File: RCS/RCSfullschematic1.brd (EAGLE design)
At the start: 102.5 x 80 mm, 67 parts, among them IC1 ILD213T, IC2 FT232RL, IC4 317T, J7 USB-MICROB, Q2 8 MHz, T1 MMBT2222A, U1 MPL3115A2, U2 MPU-9250, U3 ATMEGA328P_TQFP, U4 ADS1015

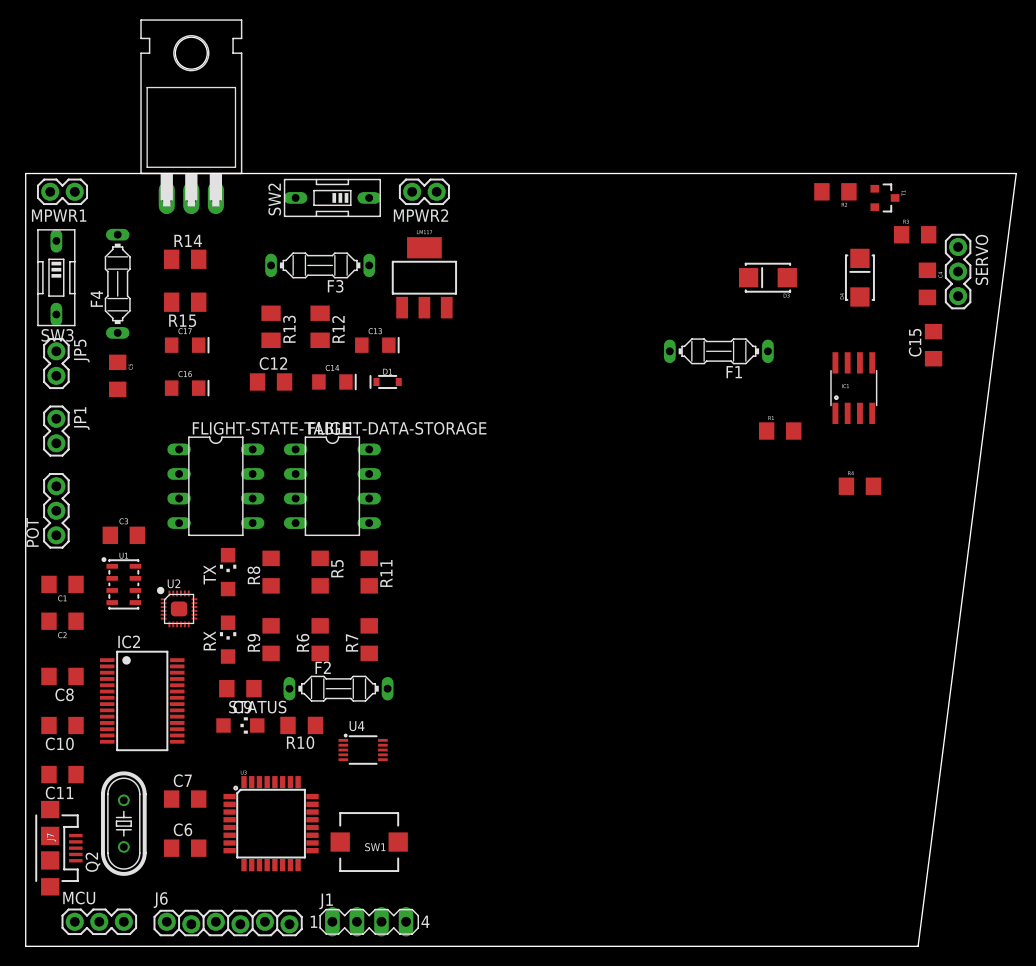
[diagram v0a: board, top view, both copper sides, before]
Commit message: Small Update to board
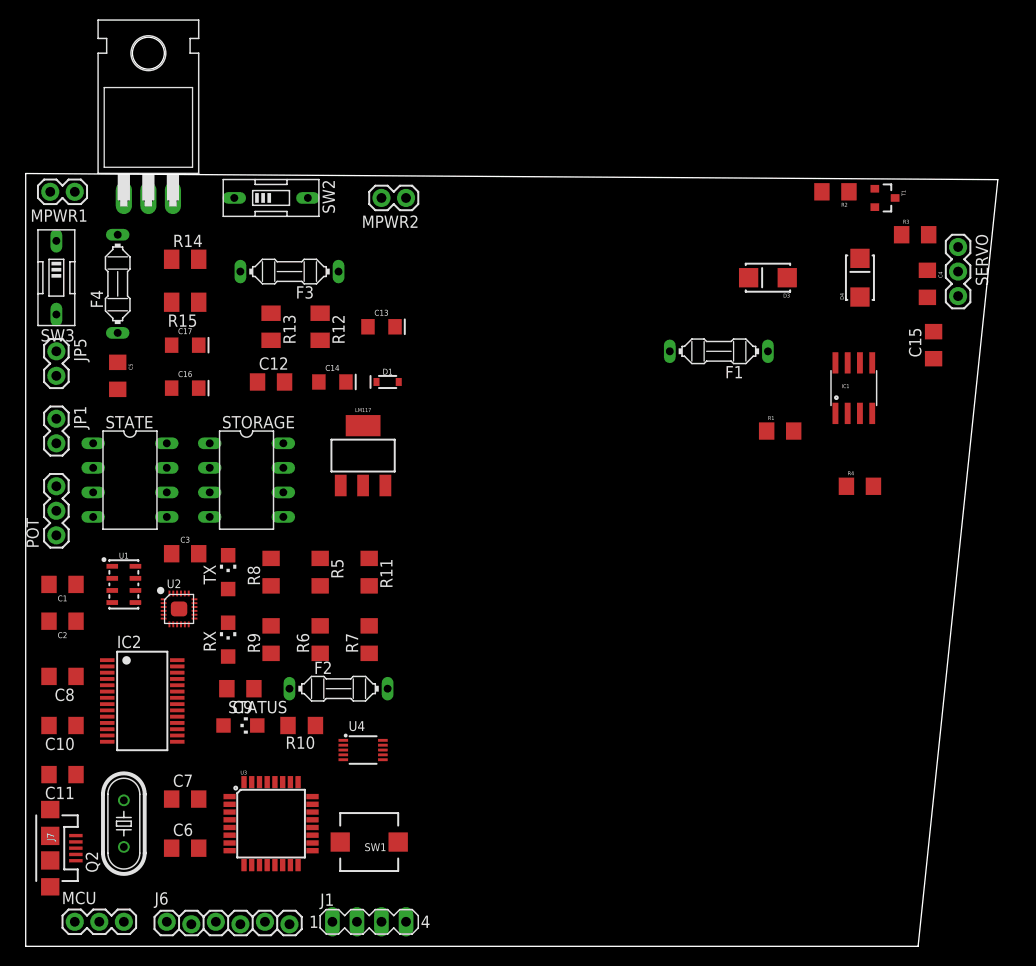
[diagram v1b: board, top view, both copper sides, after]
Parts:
- removed FLIGHT-DATA-STORAGE, FLIGHT-STATE-TABLE: AT24CP, atmel:DIL08
- added STATE, STORAGE: AT24CP, atmel:DIL08
- moved LM117 19.5 mm to (34.9, 50.8)
- moved C3 6.63 mm to (16.5, 40.6)
- moved SW2 6.35 mm to (25.4, 77.5), turned to 270 degrees
- moved IC4 4.45 mm to (12.7, 87.6)
- moved MPWR2 3.24 mm to (39.4, 77.5)
- moved F3 3.24 mm to (27.3, 69.8)
- moved C13 2.01 mm to (36.8, 64.1)
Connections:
- net A4(SDA): now also STATE.5, STORAGE.5; no longer FLIGHT-DATA-STORAGE.5, FLIGHT-STATE-TABLE.5
- net A5(SCL): now also STATE.6, STORAGE.6; no longer FLIGHT-DATA-STORAGE.6, FLIGHT-STATE-TABLE.6
- net GND: now also STATE.1, STATE.2, STATE.4, STORAGE.1, STORAGE.2, STORAGE.3, STORAGE.4, STORAGE.7; no longer FLIGHT-DATA-STORAGE.1, FLIGHT-DATA-STORAGE.2, FLIGHT-DATA-STORAGE.3, FLIGHT-DATA-STORAGE.4, FLIGHT-DATA-STORAGE.7, FLIGHT-STATE-TABLE.1, FLIGHT-STATE-TABLE.2, FLIGHT-STATE-TABLE.4
- net VCC: now also STATE.3, STATE.7, STATE.8, STORAGE.8; no longer FLIGHT-DATA-STORAGE.8, FLIGHT-STATE-TABLE.3, FLIGHT-STATE-TABLE.7, FLIGHT-STATE-TABLE.8
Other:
- board size 102.5 x 80 mm -> 100.6 x 80 mm

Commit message: yayyyyy
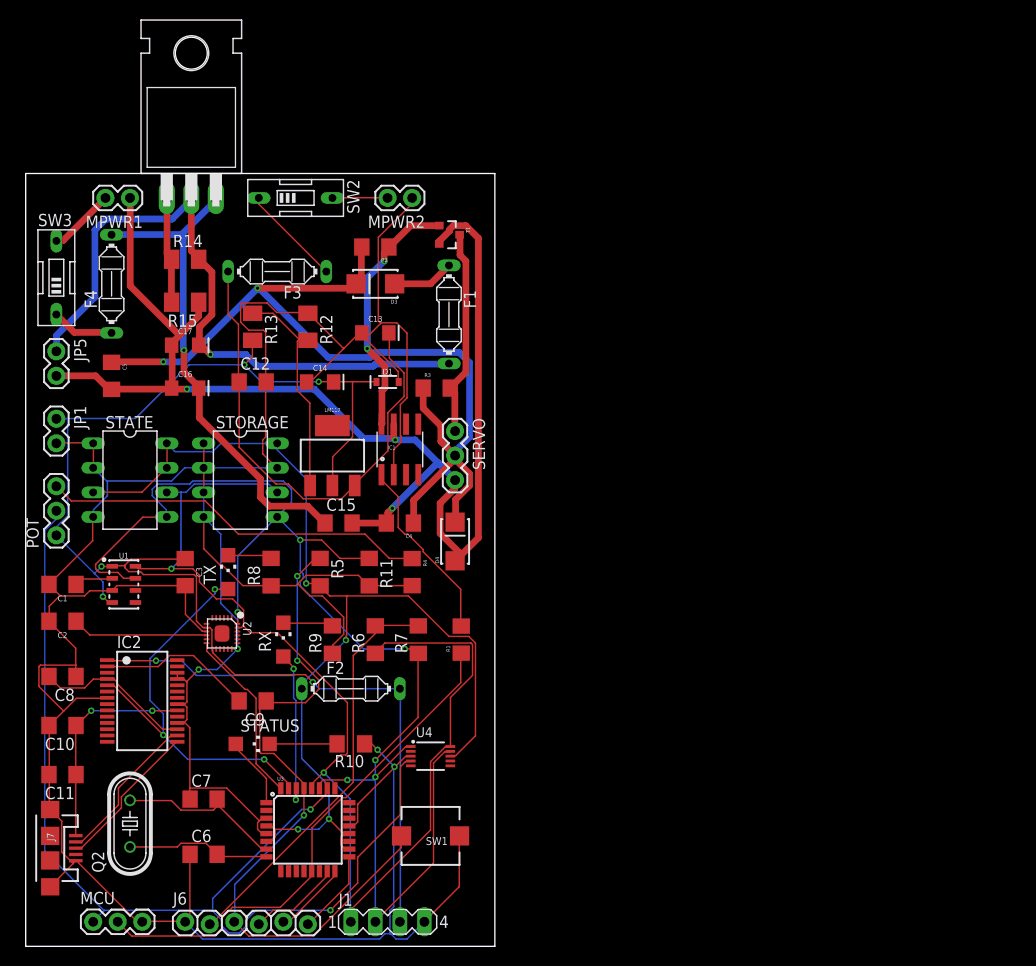
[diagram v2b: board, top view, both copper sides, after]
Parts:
- moved C15 64.3 mm to (32.4, 43.8), turned to 0 degrees
- moved C4 60.0 mm to (38.7, 43.8), turned to 180 degrees
- moved SERVO 55.4 mm to (44.5, 53.3)
- moved R3 52.0 mm to (42.5, 57.8)
- moved D4 50.0 mm to (44.5, 41.9)
- moved R2 48.0 mm to (36.2, 72.4)
- moved IC1 47.4 mm to (38.7, 51.4)
- moved R4 47.2 mm to (40.0, 38.7), turned to 270 degrees
- moved T1 45.2 mm to (43.8, 73.7)
- moved D3 40.6 mm to (36.2, 68.6)
- moved R1 39.5 mm to (45.1, 31.8), turned to 90 degrees
- moved F1 28.2 mm to (43.8, 65.4), turned to 270 degrees
- moved U4 7.01 mm to (41.9, 19.7)
- moved SW1 6.38 mm to (41.9, 11.4)
- moved R9 6.35 mm to (31.8, 31.8)
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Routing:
- net GND: track 0.00 -> 375.6 mm, vias 0 -> 4
- net LOGIC_VDD: track 0.00 -> 145.0 mm, vias 0 -> 5
- net A4(SDA): track 0.00 -> 142.9 mm, vias 0 -> 6
- net GND1: track 0.00 -> 135.8 mm, vias 0 -> 3
- net A5(SCL): track 0.00 -> 122.5 mm, vias 0 -> 2
- net VCC: track 0.00 -> 113.2 mm, vias 0 -> 4
- net FEEDBACK: track 0.00 -> 109.5 mm, vias 0 -> 2
- net 6V_POWER: track 0.00 -> 93.8 mm, vias 0 -> 2
- net RESET: track 0.00 -> 73.7 mm, vias 0 -> 3
- net VOUT-MOTOR: track 0.00 -> 69.3 mm, vias 0 -> 1
- net MOTOR: track 0.00 -> 53.7 mm
- net N$17: track 0.00 -> 52.0 mm
- net N$21: track 0.00 -> 50.9 mm, vias 0 -> 1
- net TX: track 0.00 -> 43.3 mm, vias 0 -> 3
- net VDD: track 0.00 -> 42.6 mm
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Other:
- board size 100.6 x 80 mm -> 48.6 x 80 mm
